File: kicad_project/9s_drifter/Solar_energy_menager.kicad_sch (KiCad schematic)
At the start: 16 parts, among them IC1 AEM10941-QFN

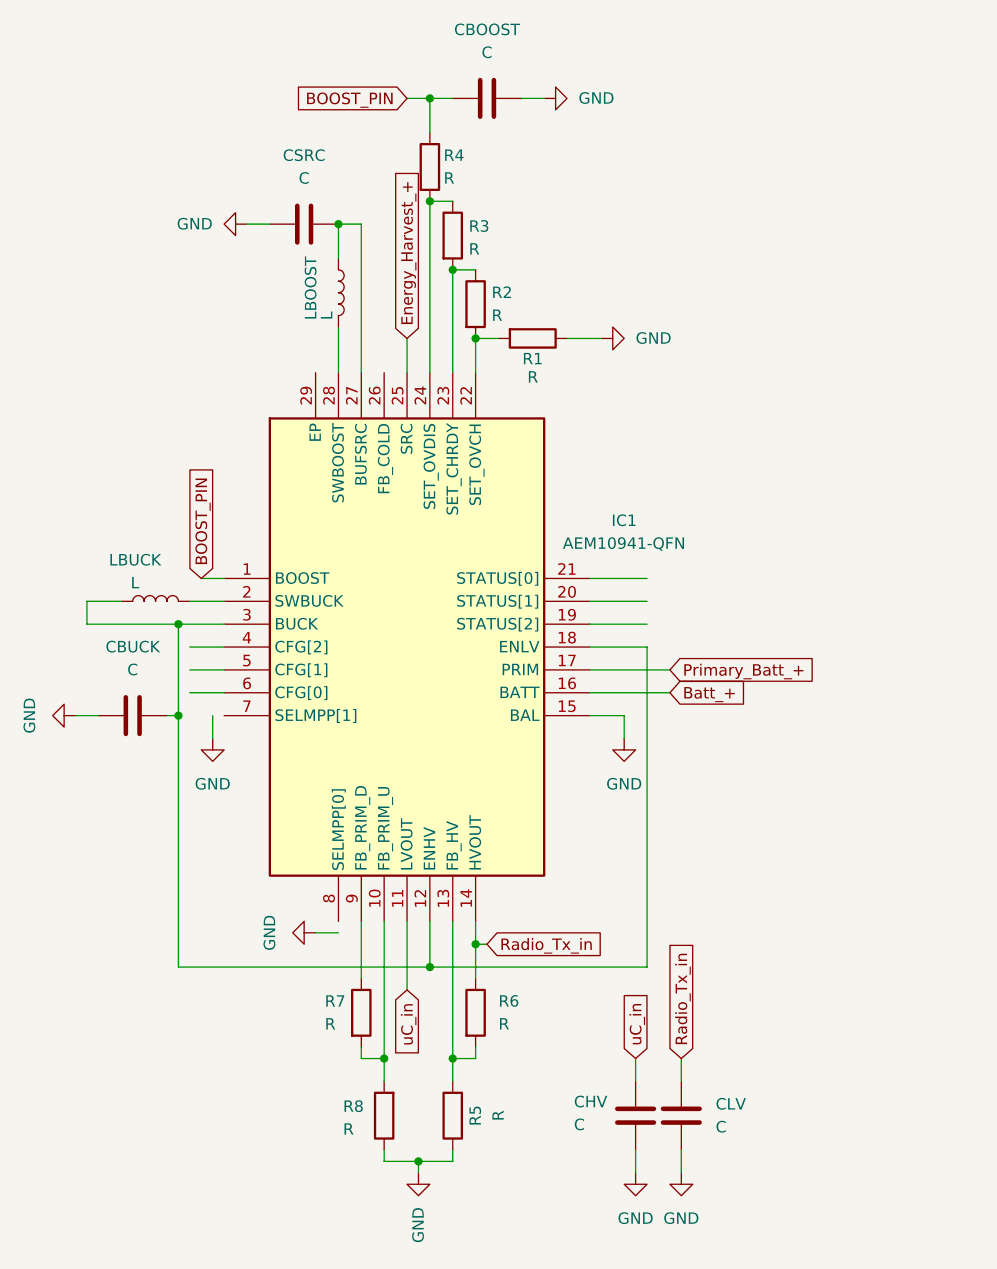
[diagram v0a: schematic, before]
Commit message: Update
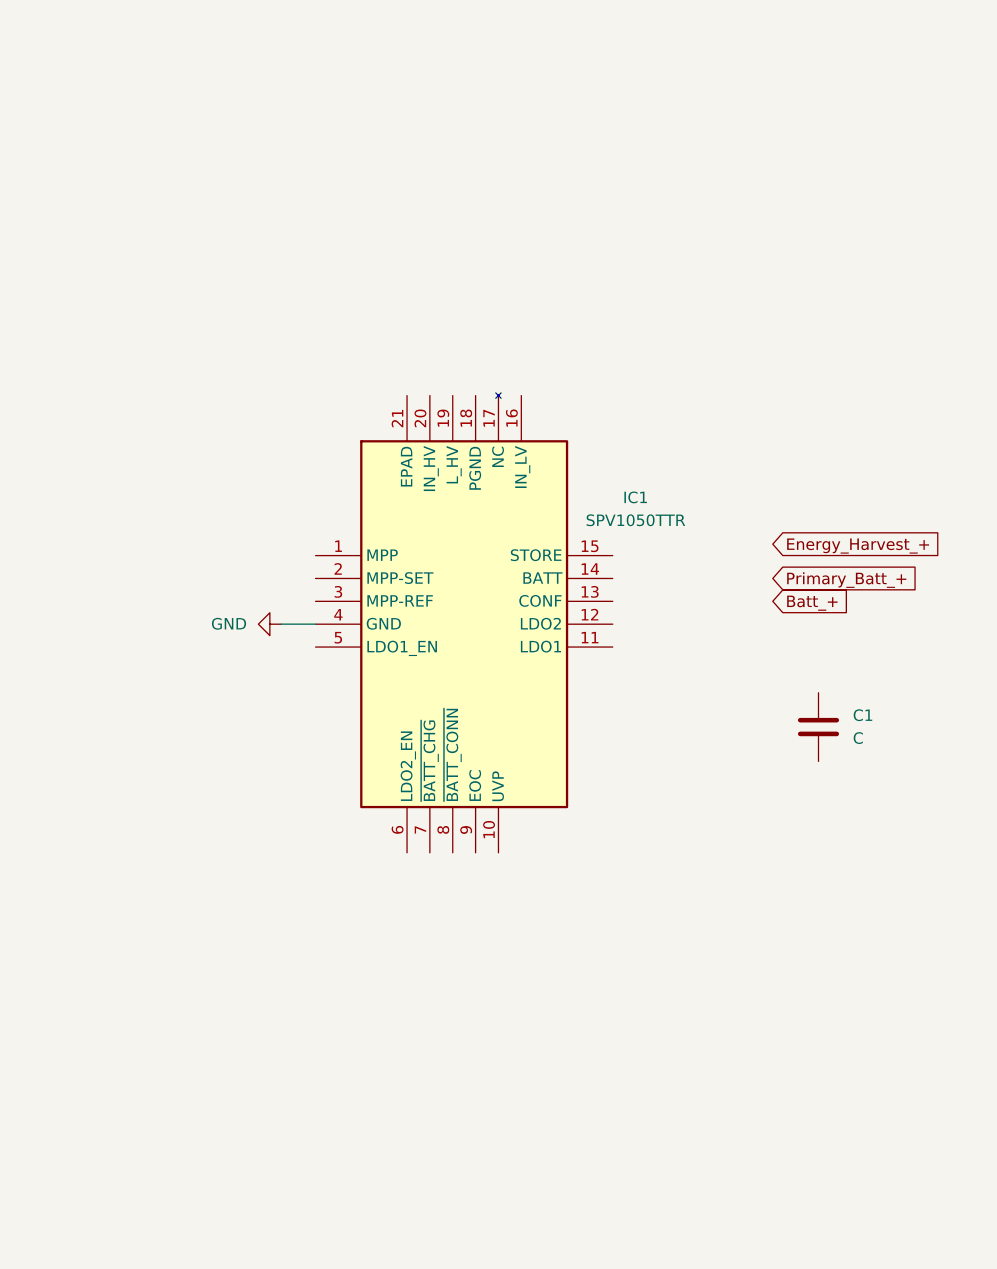
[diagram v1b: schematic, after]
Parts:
- removed CBOOST, CBUCK, CHV, CLV, CSRC: C, symbol Device:C
- removed IC1: AEM10941-QFN, QFN50P500X500X90-29N-D, symbol AEM10941:AEM10941-QFN
- removed LBOOST, LBUCK: L, symbol Device:L
- removed R1, R2, R3, R4, R5, R6, R7, R8: R, symbol Device:R
- added C1: C, symbol Device:C
- added IC1: SPV1050TTR, QFN40P300X300X100-21N-D, symbol SPV1050TTR:SPV1050TTR
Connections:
- net GND: now also IC1.4 (GND)
